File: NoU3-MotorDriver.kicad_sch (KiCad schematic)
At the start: 9 parts, among them J7 Screw_Terminal_01x02, J8 Screw_Terminal_01x02

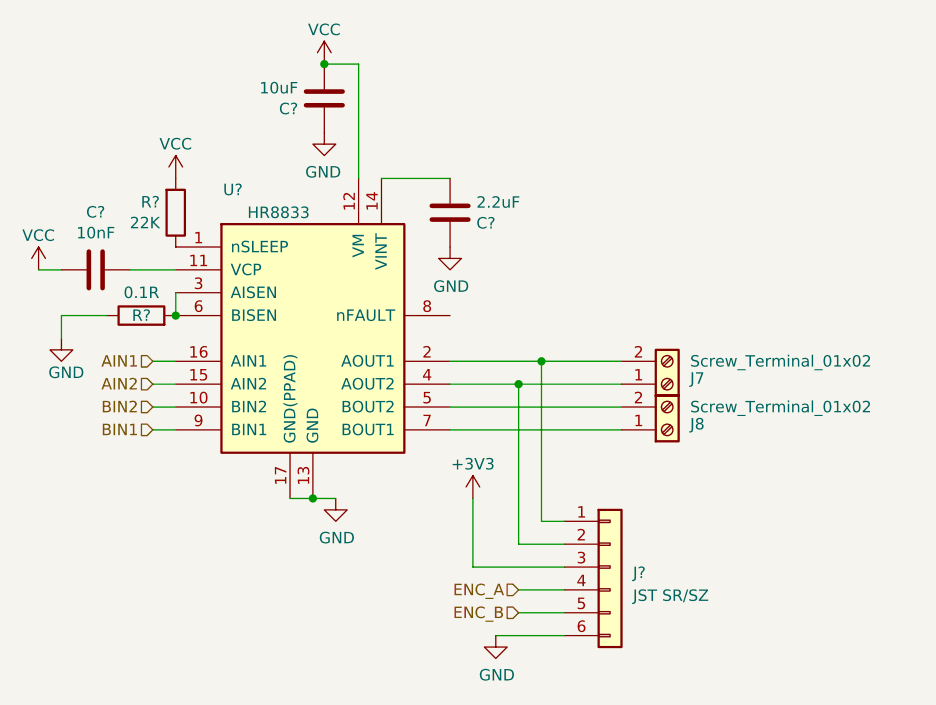
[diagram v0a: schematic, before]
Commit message: finished main changes, just need to route now
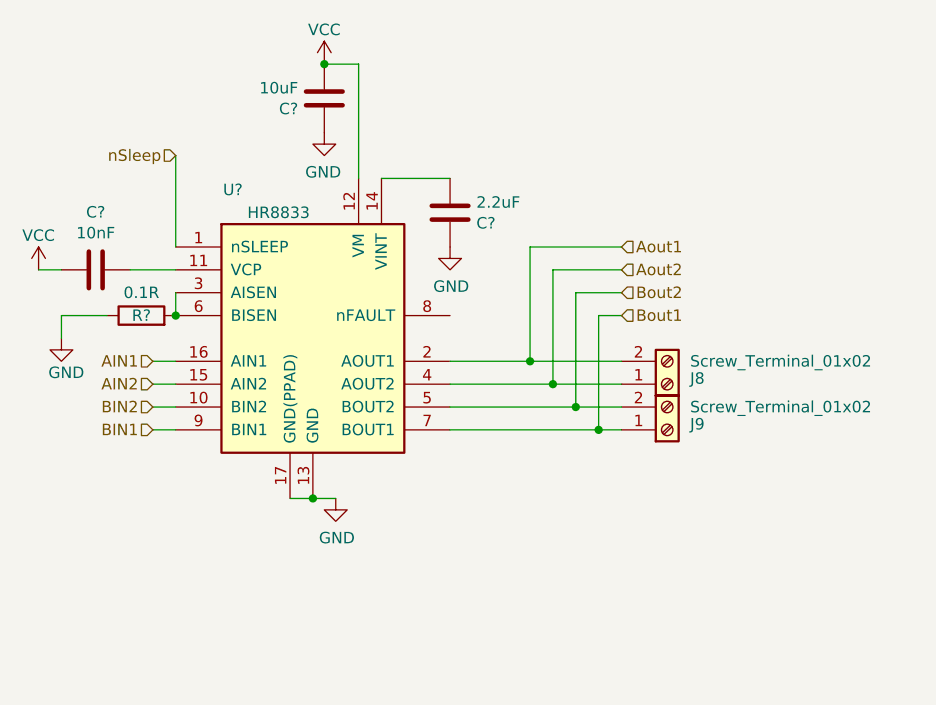
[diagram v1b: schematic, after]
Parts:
- removed J7: Screw_Terminal_01x02, AlfredoFootprints:TerminalBlock_Ningbo_2P_5mm, symbol Connector:Screw_Terminal_01x02
- removed J?: JST SR/SZ, Connector_JST:JST_SH_BM06B-SRSS-TB_1x06-1MP_P1.00mm_Vertical, symbol Connector_Generic:Conn_01x06
- removed R?: 22K, Resistor_SMD:R_0402_1005Metric, symbol Device:R
- added J9: Screw_Terminal_01x02, AlfredoFootprints:TerminalBlock_Ningbo_2P_5mm, symbol Connector:Screw_Terminal_01x02
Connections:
- net nSleep: now reaches U?.1 (nSLEEP)
- net Aout1: now reaches U?.2 (AOUT1)
- net Aout1: now also J8.2 (Pin_2)
- net Aout2: now reaches U?.4 (AOUT2)
- net Aout2: now also J8.1 (Pin_1)
- net Bout2: now reaches U?.5 (BOUT2)
- net Bout2: now also J9.2 (Pin_2); no longer J8.2 (Pin_2)
- net Bout1: now reaches U?.7 (BOUT1)
- net Bout1: now also J9.1 (Pin_1); no longer J8.1 (Pin_1)

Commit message: NoU3 as ordered 8/7/23
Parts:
- R?: LCSC C270655 -> C346796
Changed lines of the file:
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@@
       (effects (font (size 1.27 1.27)) hide)
     )
-    (property "Datasheet" "https://jlcpcb.com/partdetail/260035-0402WGF100LTCE/C270655" (at 137.16 91.44 0)
+    (property "Datasheet" "https://www.lcsc.com/product-detail/Current-Sense-Resistors-Shunt-Resistors_SEIStackpole-Elec-SEIStackpole-Elec-CSR0402FKR100_C346796.html" (at 137.16 91.44 0)
       (effects (font (size 1.27 1.27)) hide)
     )
-    (property "LCSC" "C270655" (at 137.16 91.44 0)
+    (property "LCSC" "C346796" (at 137.16 91.44 0)
       (effects (font (size 1.27 1.27)) hide)
     )
